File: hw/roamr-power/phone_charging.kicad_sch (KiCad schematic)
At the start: 12 parts, among them Q1 Q_PMOS_DSG, SW1 SW_SPDT, U2 TPS2553DDBVR

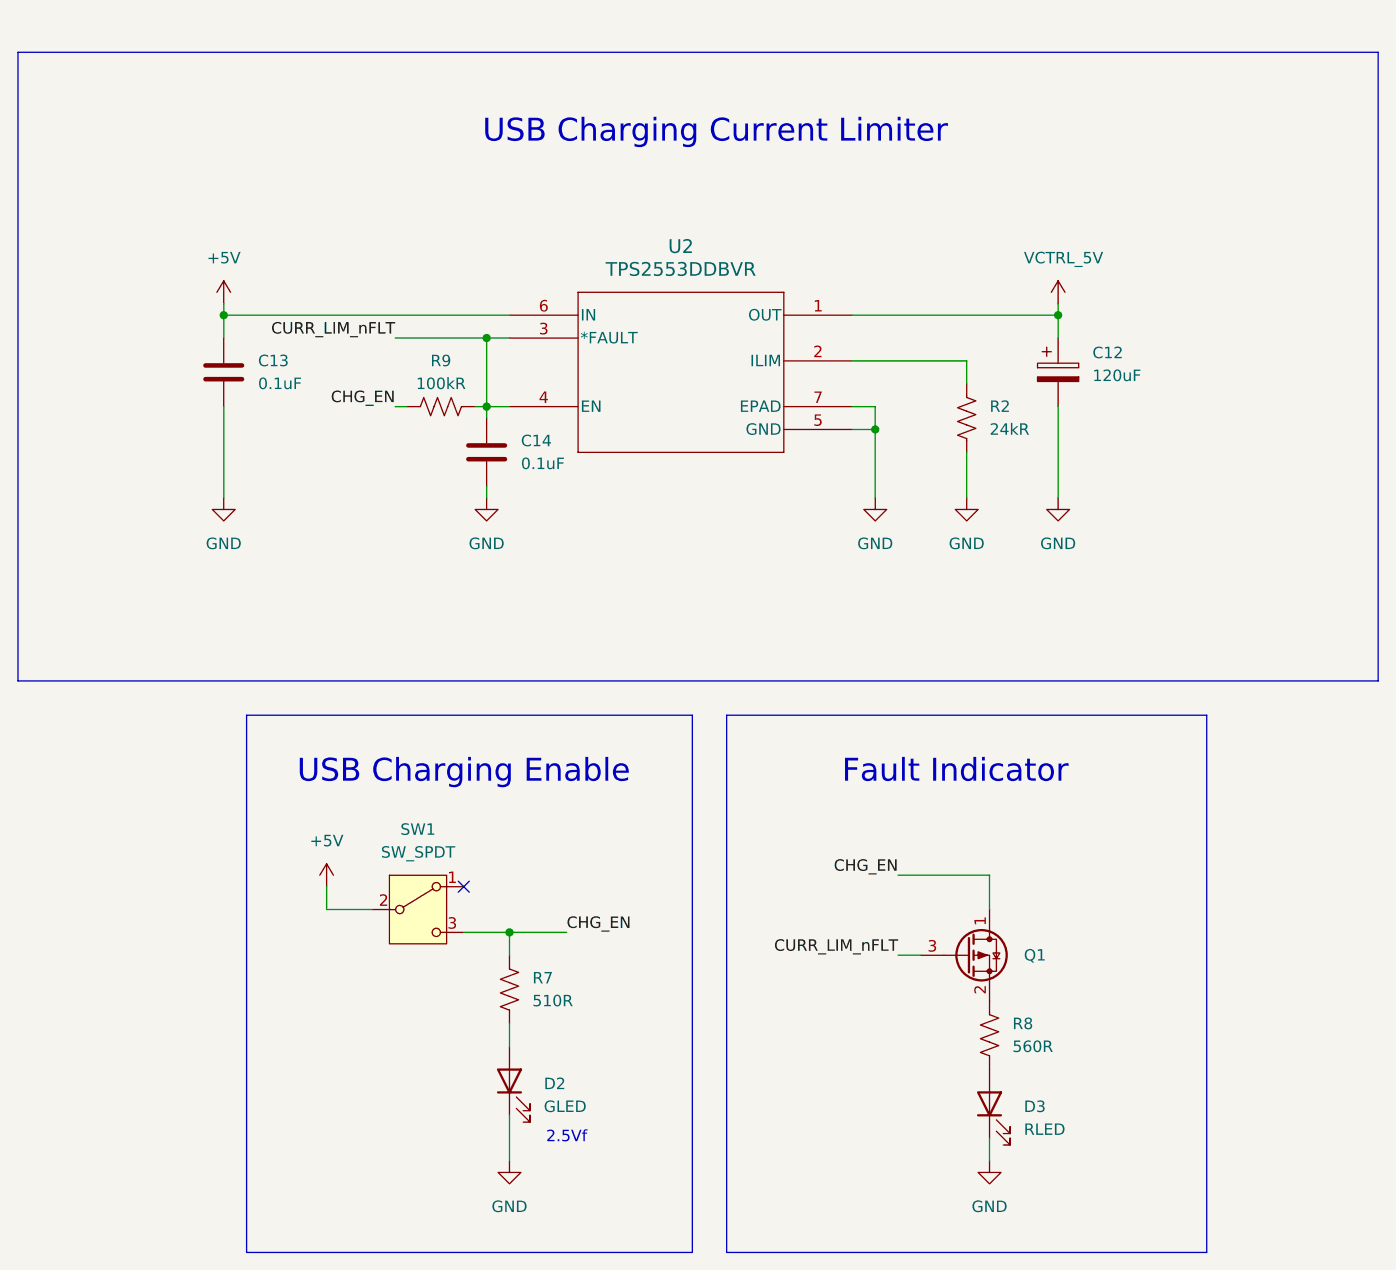
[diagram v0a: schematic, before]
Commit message: pcb schematic and layout updated
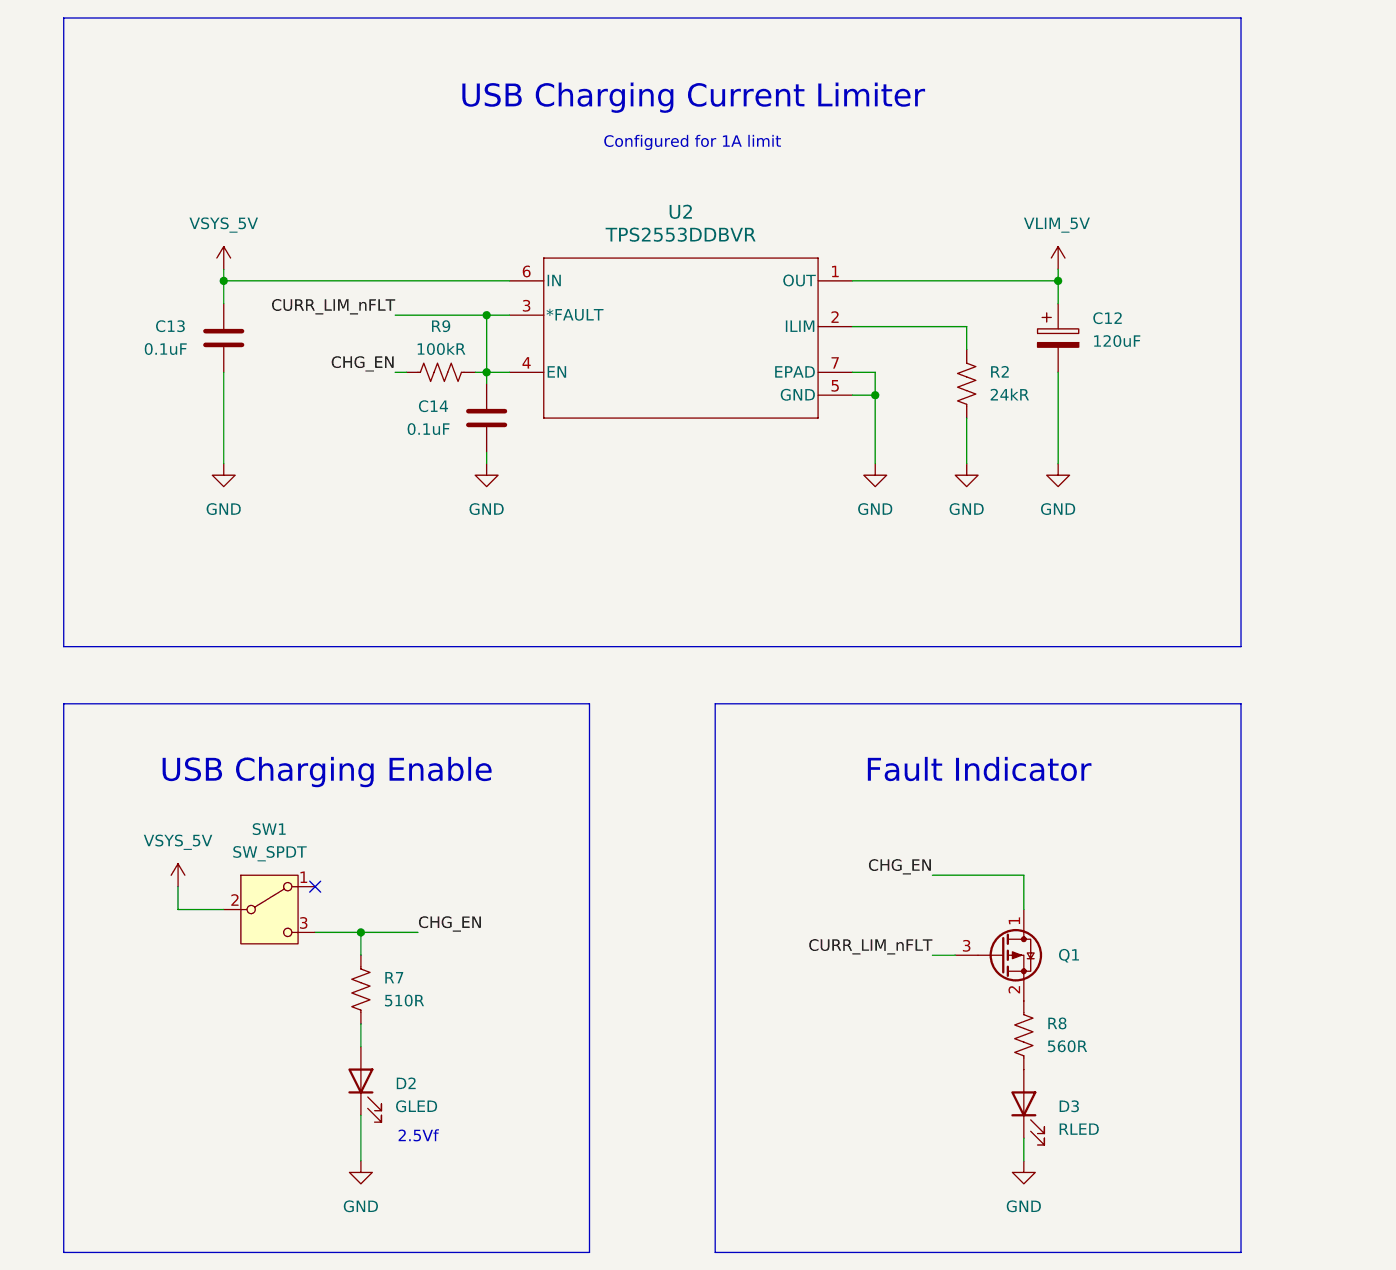
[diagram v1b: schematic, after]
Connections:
- net +5V renamed VSYS_5V
- net VCTRL_5V renamed VLIM_5V
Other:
- note added: "Configured for 1A limit"
- moved on the sheet: C12, C13, C14, D2, D3, Q1, R2, R7, R8, R9, SW1, U2
